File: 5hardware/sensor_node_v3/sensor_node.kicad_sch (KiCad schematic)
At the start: 30 parts, among them J1 Conn_01x03, J3 Conn_01x29, SW1 SW_Push, SW2 SW_DIP_x04, SW4 SW_DIP_x04, SW5 RotaryEncoder, SW6 SW_Push, U1 MCP1700x-330xxTO, U7 CH32V003F4P6, U8 ESP32-WROOM-32D

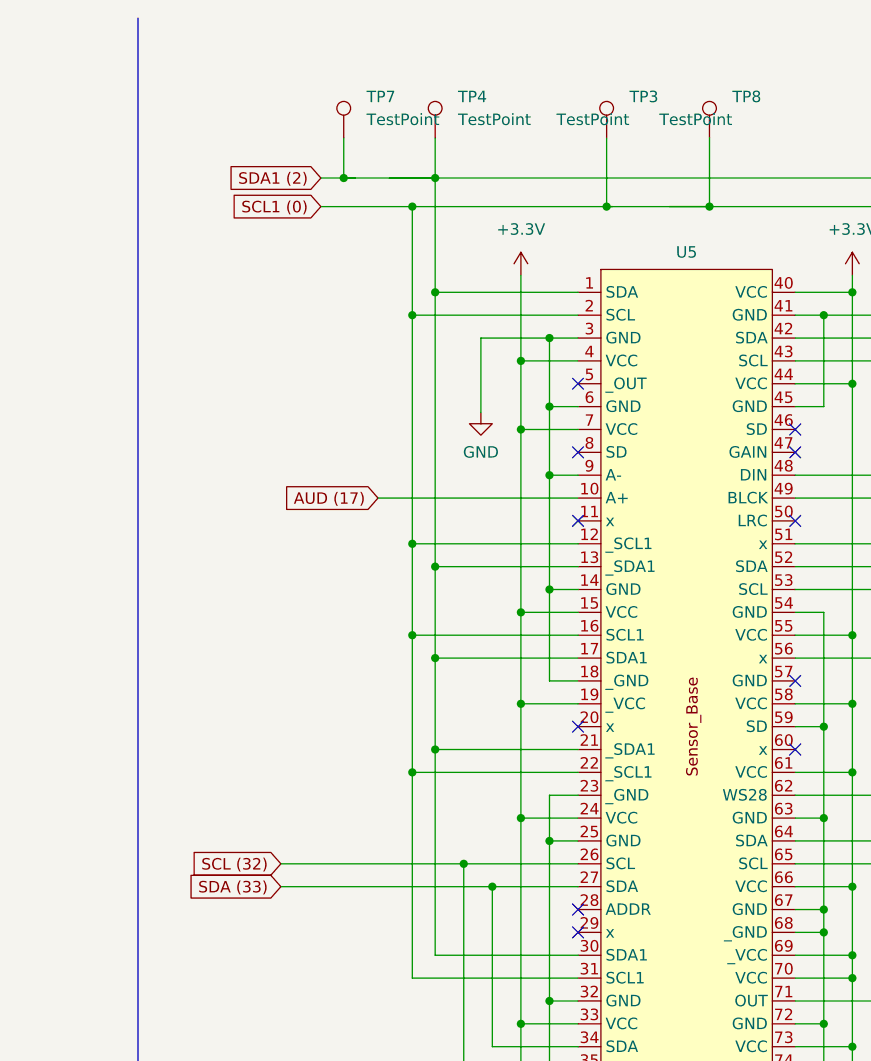
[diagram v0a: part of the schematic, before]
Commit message: fixing pcb design.
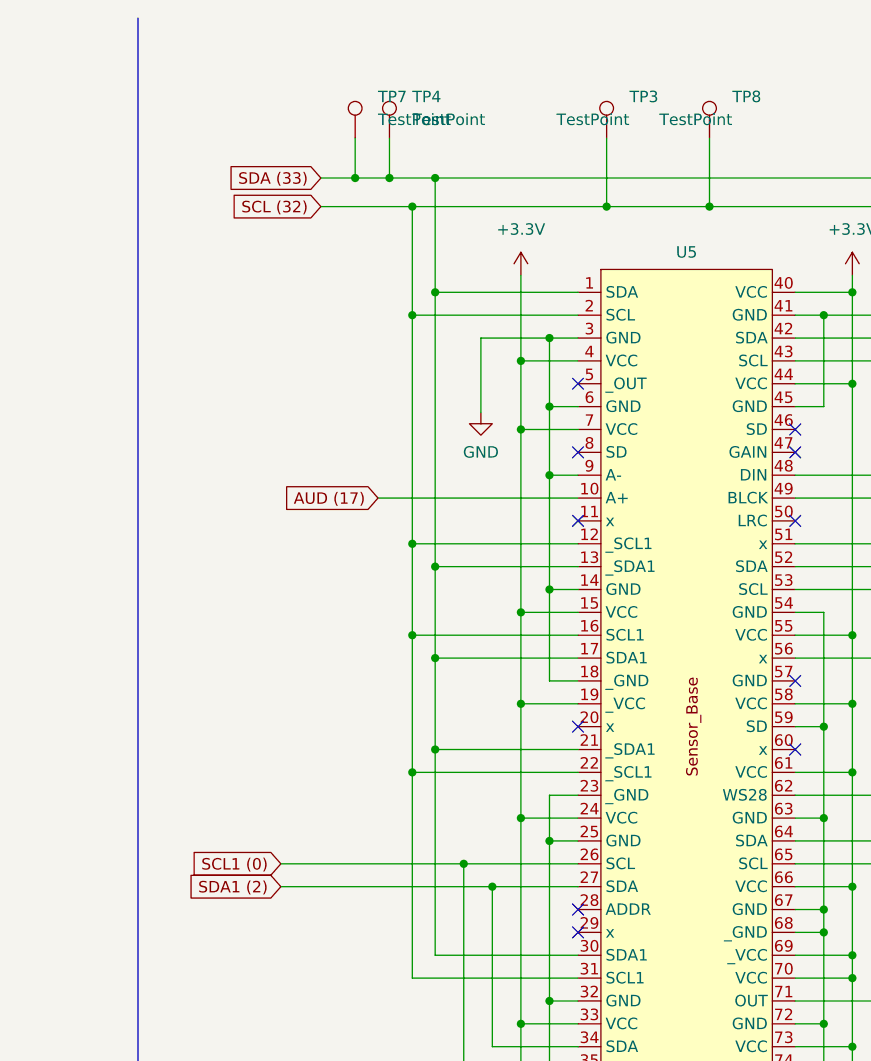
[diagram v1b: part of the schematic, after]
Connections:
- net SCL (32): now also TP3.1, TP8.1, U5.12 (_SCL1), U5.16 (SCL1), U5.2 (SCL), U5.22 (_SCL1), U5.31 (SCL1), U5.43 (SCL), U5.53 (SCL), U5.65 (SCL); no longer U5.26 (SCL), U5.35 (SCL)
- net SCL1 (0): now also U5.26 (SCL), U5.35 (SCL); no longer TP3.1, TP8.1, U5.12 (_SCL1), U5.16 (SCL1), U5.2 (SCL), U5.22 (_SCL1), U5.31 (SCL1), U5.43 (SCL), U5.53 (SCL), U5.65 (SCL)
- net SDA (33): now also TP4.1, TP7.1, U5.1 (SDA), U5.13 (_SDA1), U5.17 (SDA1), U5.21 (_SDA1), U5.30 (SDA1), U5.42 (SDA), U5.52 (SDA), U5.64 (SDA); no longer U5.27 (SDA), U5.34 (SDA)
- net SDA1 (2): now also U5.27 (SDA), U5.34 (SDA); no longer TP4.1, TP7.1, U5.1 (SDA), U5.13 (_SDA1), U5.17 (SDA1), U5.21 (_SDA1), U5.30 (SDA1), U5.42 (SDA), U5.52 (SDA), U5.64 (SDA)
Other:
- moved on the sheet: TP4, TP7
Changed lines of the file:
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@@
   (junction (at 47.625 229.87) (diameter 0) (color 0 0 0 0)
   )
-  (junction (at 351.79 33.02) (diameter 0) (color 0 0 0 0)
-  )
   (junction (at 379.095 42.545) (diameter 0) (color 0 0 0 0)
   )
@@
   (junction (at 330.2 45.085) (diameter 0) (color 194 194 194 1)
   )
+  (junction (at 323.85 29.845) (diameter 0) (color 0 0 0 0)
+  )
   (junction (at 232.41 136.525) (diameter 0) (color 0 0 0 0)
   )
@@
   (junction (at 229.87 194.945) (diameter 0) (color 255 153 0 1)
   )
-  (junction (at 322.58 29.845) (diameter 0) (color 0 0 0 0)
+  (junction (at 327.66 29.845) (diameter 0) (color 0 0 0 0)
   )
   (junction (at 332.74 42.545) (diameter 0) (color 0 0 0 1)
@@
   (junction (at 50.165 61.595) (diameter 0) (color 255 0 0 1)
   )
+  (junction (at 351.79 33.02) (diameter 0) (color 0 0 0 0)
+  )
   (junction (at 379.095 88.265) (diameter 0) (color 255 0 0 1)
   )
@@
   (no_connect (at 368.3 225.425))
   (no_connect (at 355.6 225.425))
+  (wire (pts (xy 327.66 29.845) (xy 323.85 29.845))
+    (stroke (width 0) (type default) (color 0 0 0 1))
+  )
   (wire (pts (xy 182.245 191.135) (xy 182.245 193.675))
     (stroke (width 0) (type default))
@@
     (stroke (width 0) (type default))
   )
-  (wire (pts (xy 351.79 33.02) (xy 363.22 33.02))
+  (wire (pts (xy 330.2 33.02) (xy 351.79 33.02))
     (stroke (width 0) (type default) (color 194 194 194 1))
   )
@@
     (stroke (width 0) (type default))
   )
-  (wire (pts (xy 351.79 33.02) (xy 352.425 33.02))
-    (stroke (width 0) (type default))
-  )
   (wire (pts (xy 379.095 80.645) (xy 379.095 88.265))
     (stroke (width 0) (type default) (color 255 0 0 1))
@@
     (stroke (width 0) (type default) (color 255 0 0 1))
   )
-  (wire (pts (xy 363.22 33.02) (xy 358.775 33.02))
-    (stroke (width 0) (type default))
-  )
   (wire (pts (xy 61.595 173.355) (xy 66.675 173.355))
     (stroke (width 0) (type default) (color 255 0 0 1))
@@
     (stroke (width 0) (type default))
   )
-  (wire (pts (xy 322.58 29.845) (xy 320.04 29.845))
-    (stroke (width 0) (type default) (color 0 0 0 1))
-  )
   (wire (pts (xy 325.12 194.945) (xy 325.12 187.96))
     (stroke (width 0) (type default) (color 194 194 194 1))
@@
     (stroke (width 0) (type default) (color 255 0 0 1))
   )
-  (wire (pts (xy 322.58 25.4) (xy 322.58 29.845))
+  (wire (pts (xy 323.85 25.4) (xy 323.85 29.845))
     (stroke (width 0) (type default))
   )
@@
     (stroke (width 0) (type default) (color 194 0 194 1))
   )
-  (wire (pts (xy 332.74 29.845) (xy 327.66 29.845))
-    (stroke (width 0) (type default))
-  )
   (wire (pts (xy 228.6 91.44) (xy 240.665 91.44))
     (stroke (width 0) (type default) (color 194 0 194 1))
@@
     (stroke (width 0) (type default) (color 255 153 0 1))
   )
-  (wire (pts (xy 322.58 29.845) (xy 332.74 29.845))
+  (wire (pts (xy 332.74 29.845) (xy 327.66 29.845))
     (stroke (width 0) (type default) (color 0 0 0 1))
   )
@@
     (stroke (width 0) (type default))
   )
-  (wire (pts (xy 322.58 29.845) (xy 323.85 29.845))
-    (stroke (width 0) (type default))
-  )
   (wire (pts (xy 375.92 45.085) (xy 388.62 45.085))
     (stroke (width 0) (type default))
@@
     (stroke (width 0) (type default) (color 194 0 194 1))
   )
-  (wire (pts (xy 332.74 25.4) (xy 332.74 29.845))
+  (wire (pts (xy 327.66 25.4) (xy 327.66 29.845))
     (stroke (width 0) (type default))
   )
@@
     (stroke (width 0) (type default))
   )
+  (wire (pts (xy 323.85 29.845) (xy 320.04 29.845))
+    (stroke (width 0) (type default) (color 0 0 0 1))
+  )
   (wire (pts (xy 23.495 114.935) (xy 35.56 114.935))
     (stroke (width 0) (type default) (color 255 0 0 1))
@@
     (stroke (width 0) (type default) (color 194 0 194 1))
   )
-  (wire (pts (xy 330.2 33.02) (xy 351.79 33.02))
-    (stroke (width 0) (type default) (color 194 194 194 1))
-  )
   (wire (pts (xy 128.27 217.17) (xy 128.27 224.155))
     (stroke (width 0) (type default))
@@
     (stroke (width 0) (type default))
   )
+  (wire (pts (xy 351.79 33.02) (xy 363.22 33.02))
+    (stroke (width 0) (type default) (color 194 194 194 1))
+  )
   (wire (pts (xy 228.6 88.9) (xy 240.665 88.9))
     (stroke (width 0) (type default) (color 194 0 194 1))
@@
     )
   )
-  (global_label "SDA (33)" (shape input) (at 315.595 108.585 180) (fields_autoplaced)
+  (global_label "SDA (33)" (shape input) (at 320.04 29.845 180) (fields_autoplaced)
     (effects (font (size 1.27 1.27)) (justify right))
-    (property "Intersheetrefs" "${INTERSHEET_REFS}" (at 303.9617 108.585 0)
+    (property "Intersheetrefs" "${INTERSHEET_REFS}" (at 308.4067 29.845 0)
       (effects (font (size 1.27 1.27)) (justify right) hide)
     )
@@
     )
   )
-  (global_label "SDA1 (2)" (shape input) (at 320.04 29.845 180) (fields_autoplaced)
+  (global_label "SDA1 (2)" (shape input) (at 315.595 108.585 180) (fields_autoplaced)
     (effects (font (size 1.27 1.27)) (justify right))
-    (property "Intersheetrefs" "${INTERSHEET_REFS}" (at 308.4067 29.845 0)
+    (property "Intersheetrefs" "${INTERSHEET_REFS}" (at 303.9617 108.585 0)
       (effects (font (size 1.27 1.27)) (justify right) hide)
     )
@@
     )
   )
-  (global_label "SCL1 (0)" (shape input) (at 320.04 33.02 180) (fields_autoplaced)
+  (global_label "SCL1 (0)" (shape input) (at 315.595 106.045 180) (fields_autoplaced)
     (effects (font (size 1.27 1.27)) (justify right))
-    (property "Intersheetrefs" "${INTERSHEET_REFS}" (at 308.4672 33.02 0)
+    (property "Intersheetrefs" "${INTERSHEET_REFS}" (at 304.0222 106.045 0)
       (effects (font (size 1.27 1.27)) (justify right) hide)
     )
@@
     )
   )
-  (global_label "SCL (32)" (shape input) (at 315.595 106.045 180) (fields_autoplaced)
+  (global_label "SCL (32)" (shape input) (at 320.04 33.02 180) (fields_autoplaced)
     (effects (font (size 1.27 1.27)) (justify right))
-    (property "Intersheetrefs" "${INTERSHEET_REFS}" (at 304.0222 106.045 0)
+    (property "Intersheetrefs" "${INTERSHEET_REFS}" (at 308.4672 33.02 0)
       (effects (font (size 1.27 1.27)) (justify right) hide)
     )
@@
     )
   )
-  (symbol (lib_id "Connector:TestPoint") (at 332.74 25.4 0) (unit 1)
+  (symbol (lib_id "Connector:TestPoint") (at 327.66 25.4 0) (unit 1)
     (in_bom yes) (on_board yes) (dnp no) (fields_autoplaced)
-    (property "Reference" "TP4" (at 335.28 20.828 0)
+    (property "Reference" "TP4" (at 330.2 20.828 0)
       (effects (font (size 1.27 1.27)) (justify left))
     )
-    (property "Value" "TestPoint" (at 335.28 23.368 0)
+    (property "Value" "TestPoint" (at 330.2 23.368 0)
       (effects (font (size 1.27 1.27)) (justify left))
     )
-    (property "Footprint" "TestPoint:TestPoint_Pad_1.5x1.5mm" (at 337.82 25.4 0)
+    (property "Footprint" "TestPoint:TestPoint_Pad_1.5x1.5mm" (at 332.74 25.4 0)
       (effects (font (size 1.27 1.27)) hide)
     )
-    (property "Datasheet" "~" (at 337.82 25.4 0)
+    (property "Datasheet" "~" (at 332.74 25.4 0)
       (effects (font (size 1.27 1.27)) hide)
     )
@@
     )
   )
-  (symbol (lib_id "Connector:TestPoint") (at 322.58 25.4 0) (unit 1)
+  (symbol (lib_id "Connector:TestPoint") (at 323.85 25.4 0) (unit 1)
     (in_bom yes) (on_board yes) (dnp no) (fields_autoplaced)
-    (property "Reference" "TP7" (at 325.12 20.828 0)
+    (property "Reference" "TP7" (at 326.39 20.828 0)
       (effects (font (size 1.27 1.27)) (justify left))
     )
-    (property "Value" "TestPoint" (at 325.12 23.368 0)
+    (property "Value" "TestPoint" (at 326.39 23.368 0)
       (effects (font (size 1.27 1.27)) (justify left))
     )
-    (property "Footprint" "TestPoint:TestPoint_Pad_1.5x1.5mm" (at 327.66 25.4 0)
+    (property "Footprint" "TestPoint:TestPoint_Pad_1.5x1.5mm" (at 328.93 25.4 0)
       (effects (font (size 1.27 1.27)) hide)
     )
-    (property "Datasheet" "~" (at 327.66 25.4 0)
+    (property "Datasheet" "~" (at 328.93 25.4 0)
       (effects (font (size 1.27 1.27)) hide)
     )
